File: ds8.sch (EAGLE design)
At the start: 87 parts, among them IC1 TM4C1230C3PM, IC2 TPS77333, Q1 BC850, Q2 BC850, Q3 BC850, U1 LM13700M, U2 LM324, U3 LM324, U4 LM741D

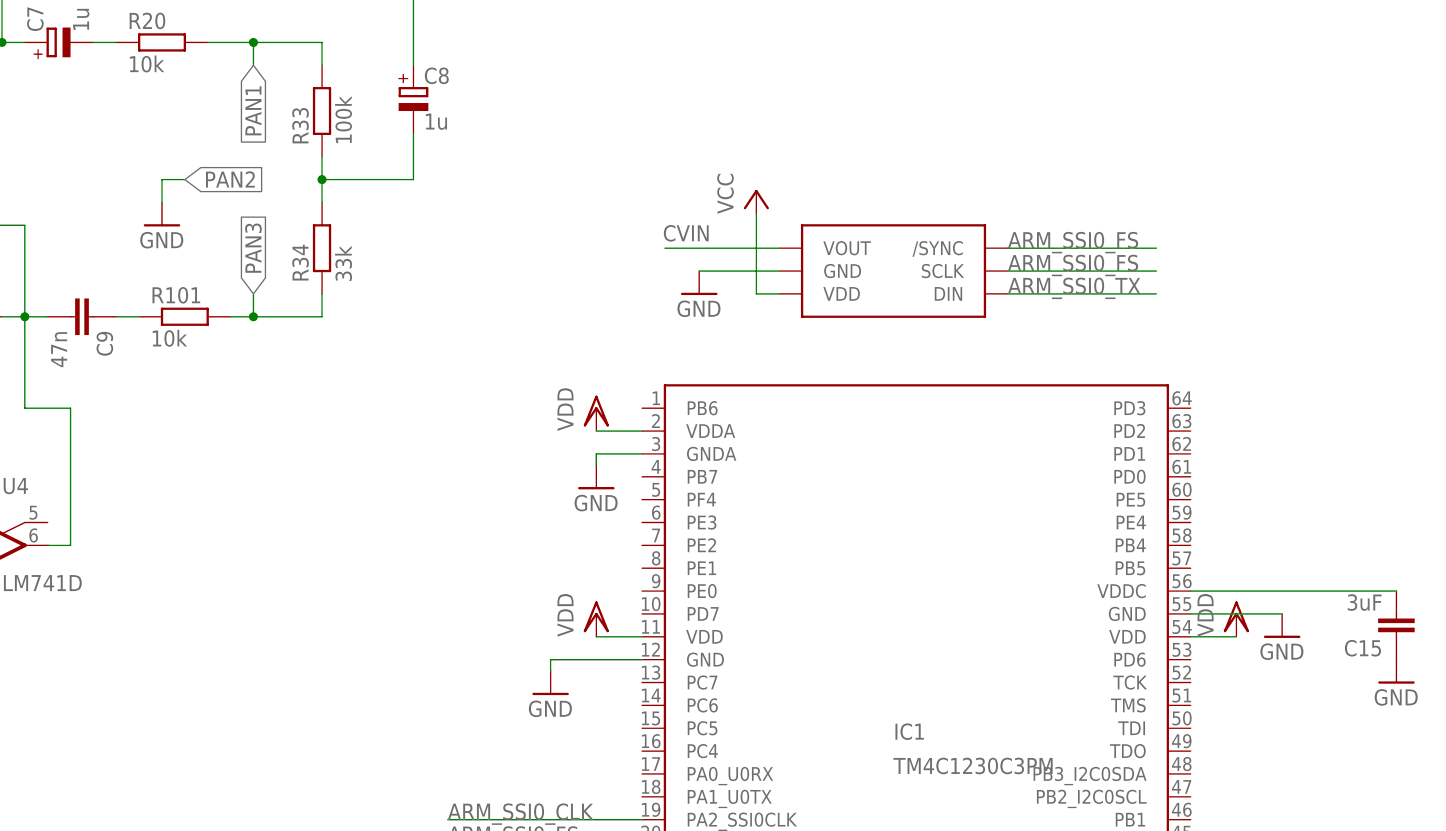
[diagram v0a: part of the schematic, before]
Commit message: wire conflicts
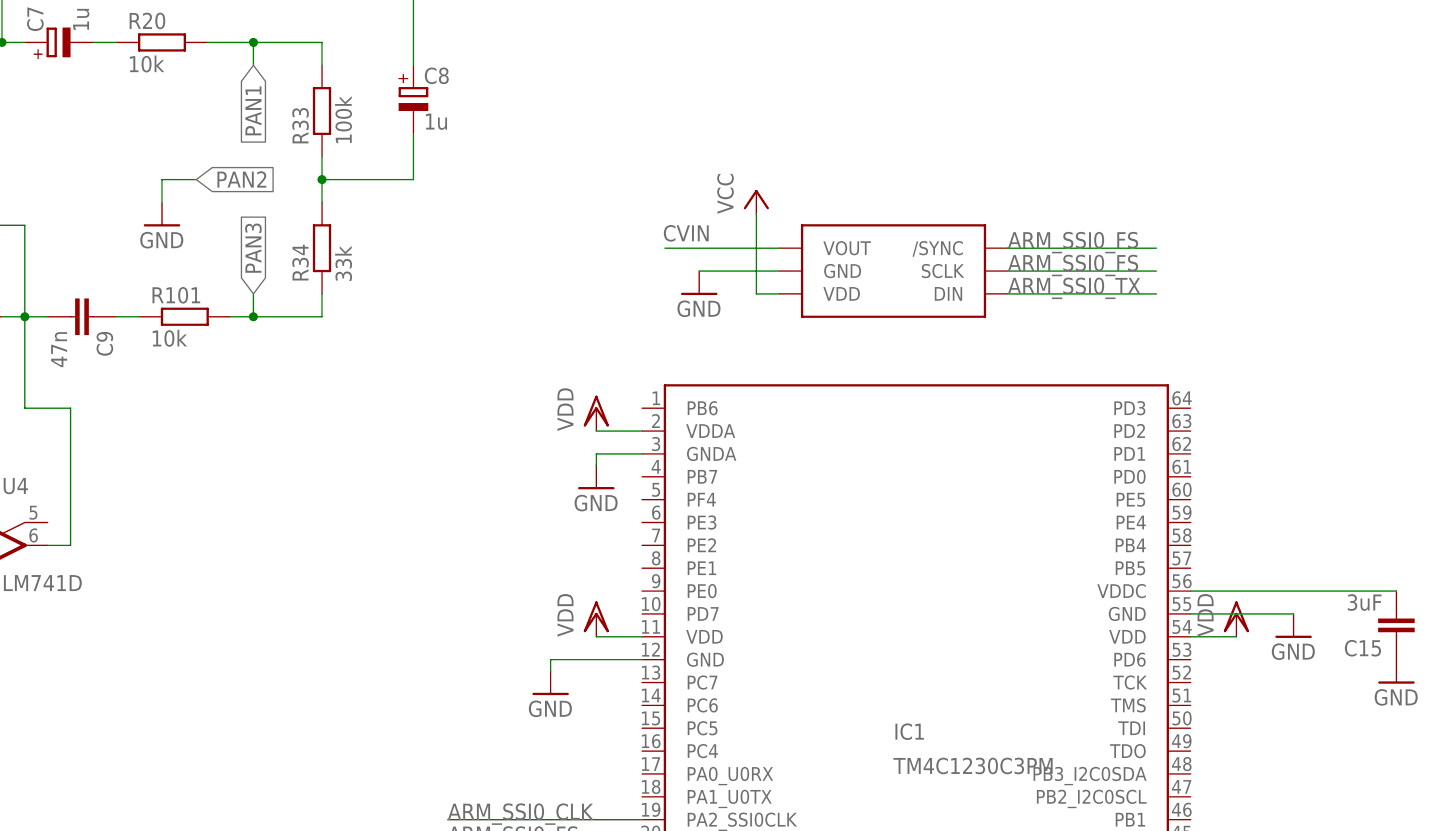
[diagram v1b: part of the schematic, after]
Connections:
- net GND: now also IC1.GND@1
- net N$36: now also IC1.VDDC@1
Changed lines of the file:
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@@
 <instance part="VDD6" gate="G$1" x="259.08" y="-129.54"/>
 <instance part="GND38" gate="1" x="254" y="-138.43"/>
-<instance part="GND39" gate="1" x="335.28" y="-132.08"/>
+<instance part="GND39" gate="1" x="336.55" y="-132.08"/>
 <instance part="GND40" gate="1" x="342.9" y="-172.72"/>
 </instances>
@@
 <pinref part="GND36" gate="1" pin="GND"/>
 <wire x1="256.54" y1="-172.72" x2="256.54" y2="-175.26" width="0.1524" layer="91"/>
+<pinref part="IC1" gate="G$1" pin="GND@1"/>
 </segment>
 <segment>
@@
 <pinref part="IC1" gate="G$1" pin="GND@3"/>
 <pinref part="GND39" gate="1" pin="GND"/>
-<wire x1="325.12" y1="-129.54" x2="335.28" y2="-129.54" width="0.1524" layer="91"/>
+<wire x1="325.12" y1="-129.54" x2="336.55" y2="-129.54" width="0.1524" layer="91"/>
 </segment>
 <segment>
@@
 <net name="PAN2" class="0">
 <segment>
-<wire x1="213.36" y1="-81.28" x2="210.82" y2="-81.28" width="0.1524" layer="91"/>
+<wire x1="214.63" y1="-81.28" x2="210.82" y2="-81.28" width="0.1524" layer="91"/>
 <wire x1="210.82" y1="-81.28" x2="210.82" y2="-83.82" width="0.1524" layer="91"/>
-<label x="213.36" y="-81.28" size="1.778" layer="95" xref="yes"/>
+<label x="214.63" y="-81.28" size="1.778" layer="95" xref="yes"/>
 <pinref part="GND11" gate="1" pin="GND"/>
 </segment>
@@
 <pinref part="C15" gate="G$1" pin="2"/>
 <wire x1="325.12" y1="-127" x2="347.98" y2="-127" width="0.1524" layer="91"/>
+<pinref part="IC1" gate="G$1" pin="VDDC@1"/>
 </segment>
 </net>
@@
 </sheet>
 </sheets>
+<errors>
+</errors>
 </schematic>
 </drawing>
